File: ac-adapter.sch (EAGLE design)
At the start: 68 parts, among them IC1 SSC3S900, IC2 TL431, Q1 300V5A, Q2 300V5A, Q3 TLP621-1, T1 COMMON_FILTER-SU10VFC, T2 TRANSFORMAER_FLYBACK-PQ2620, T3 COMMON_FILTER-SMALL

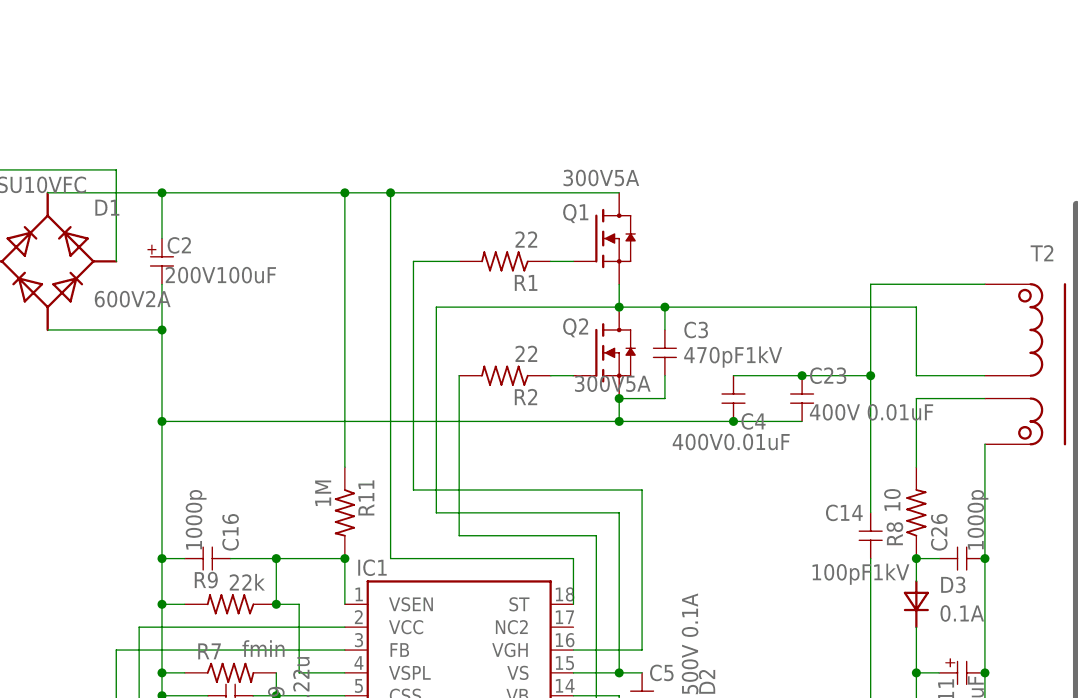
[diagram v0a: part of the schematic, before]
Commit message: 微修正
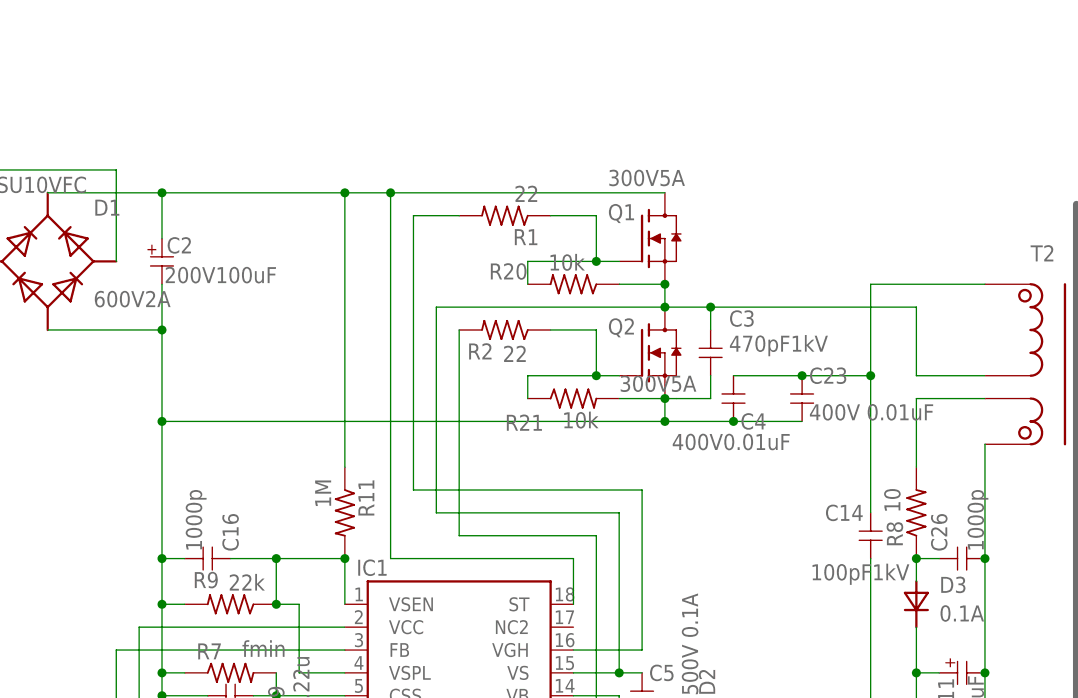
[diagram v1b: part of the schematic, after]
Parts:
- added R20, R21: 10k, my_rcl:R-1608
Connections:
- removed net N$11: Q2.G, R2.1
- removed net N$9: Q1.G, R1.1
- new net N$38: Q1.G, R1.1, R20.2
- new net N$39: Q2.G, R2.1, R21.1
- net PGND: now also R21.2
- net SW: now also R20.1
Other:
- moved on the sheet: C3, Q1, Q2, R1, R2
